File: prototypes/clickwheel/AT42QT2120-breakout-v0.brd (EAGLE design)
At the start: 26.6 x 16.2 mm, 5 parts

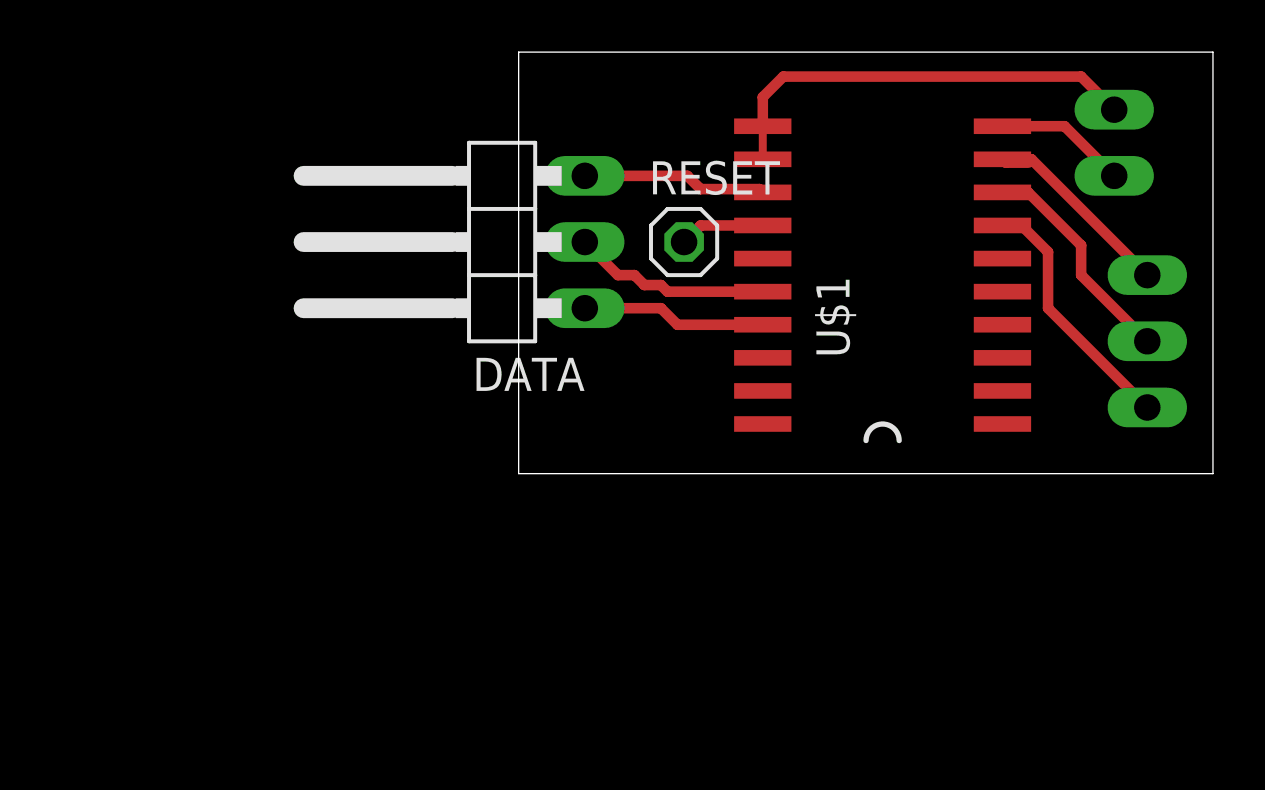
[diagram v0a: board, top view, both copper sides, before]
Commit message: update ATQ breakouts
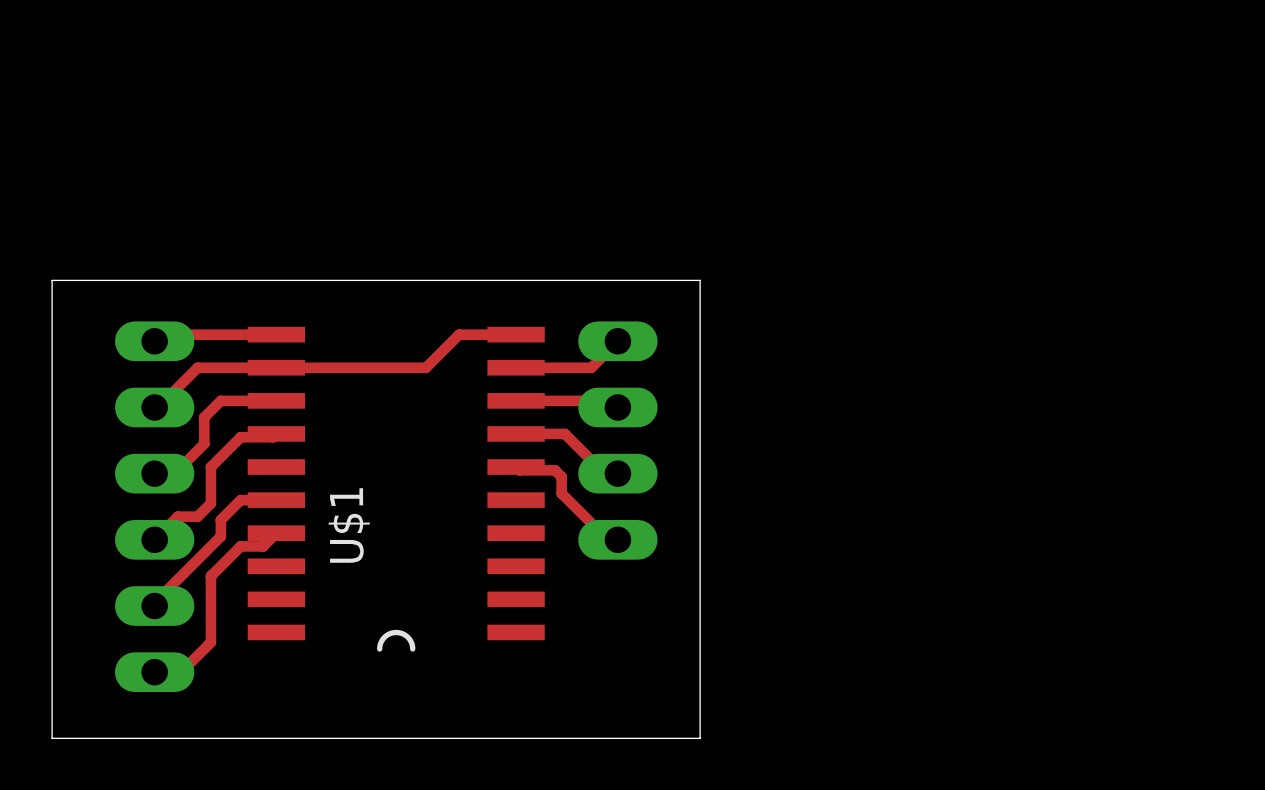
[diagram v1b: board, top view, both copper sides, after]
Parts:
- removed CLICKWHEEL, DATA: (no value), pinhead:1X03/90
- removed RESET: (no value), pinhead:1X01
- added CONTROL, JP1: (no value), pinhead:1X04/90
- moved POWER 45.3 mm to (2.54, 16.5), turned to 270 degrees
- moved U$1 20.3 mm to (15.6, 12.3)
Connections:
- removed net N$1: RESET.1, U$1.14
- removed net N$2: DATA.1, U$1.17
- removed net N$4: DATA.2, U$1.16
- removed net N$8: DATA.3, U$1.13
- new net CHANGE: CONTROL.4, U$1.17
- new net N$3: JP1.1, U$1.6
- new net RESET: CONTROL.2, U$1.14
- new net SCL: CONTROL.3, U$1.16
- new net SDA: CONTROL.1, U$1.13
- net GND: now also U$1.10; no longer U$1.11
- net N$5: now also JP1.4; no longer CLICKWHEEL.3
- net N$6: now also JP1.3; no longer CLICKWHEEL.2
- net N$7: now also JP1.2; no longer CLICKWHEEL.1
- net V3P3: now also U$1.11; no longer U$1.10
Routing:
- net CHANGE: track 0.00 -> 8.37 mm
- net N$4: track 7.62 -> 0.00 mm
- net SDA: track 0.00 -> 7.41 mm
- net RESET: track 0.00 -> 7.17 mm
- net N$2: track 7.09 -> 0.00 mm
- net N$8: track 7.09 -> 0.00 mm
- net SCL: track 0.00 -> 6.80 mm
- net N$3: track 0.00 -> 5.44 mm
- net N$7: track 9.72 -> 4.54 mm
- net N$6: track 8.60 -> 4.01 mm
- net N$5: track 8.44 -> 4.33 mm
- net N$1: track 3.28 -> 0.00 mm
- net GND: track 16.7 -> 15.0 mm
- net V3P3: track 6.19 -> 4.78 mm
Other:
- board size 26.6 x 16.2 mm -> 24.9 x 17.6 mm

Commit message: update ATQ prototype board files
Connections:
- net N$5 renamed KEY0
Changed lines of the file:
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@@
 <wire x1="6.477" y1="15.24" x2="6.35" y2="15.24" width="0.4064" layer="1"/>
 </signal>
-<signal name="N$5">
+<signal name="KEY0">
 <contactref element="U$1" pad="9"/>
 <contactref element="JP1" pad="4"/>
